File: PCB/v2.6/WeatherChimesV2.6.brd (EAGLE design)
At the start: 102.8 x 78.9 mm, 31 parts, among them U1 MS5803-02BA, X4 BQ24074

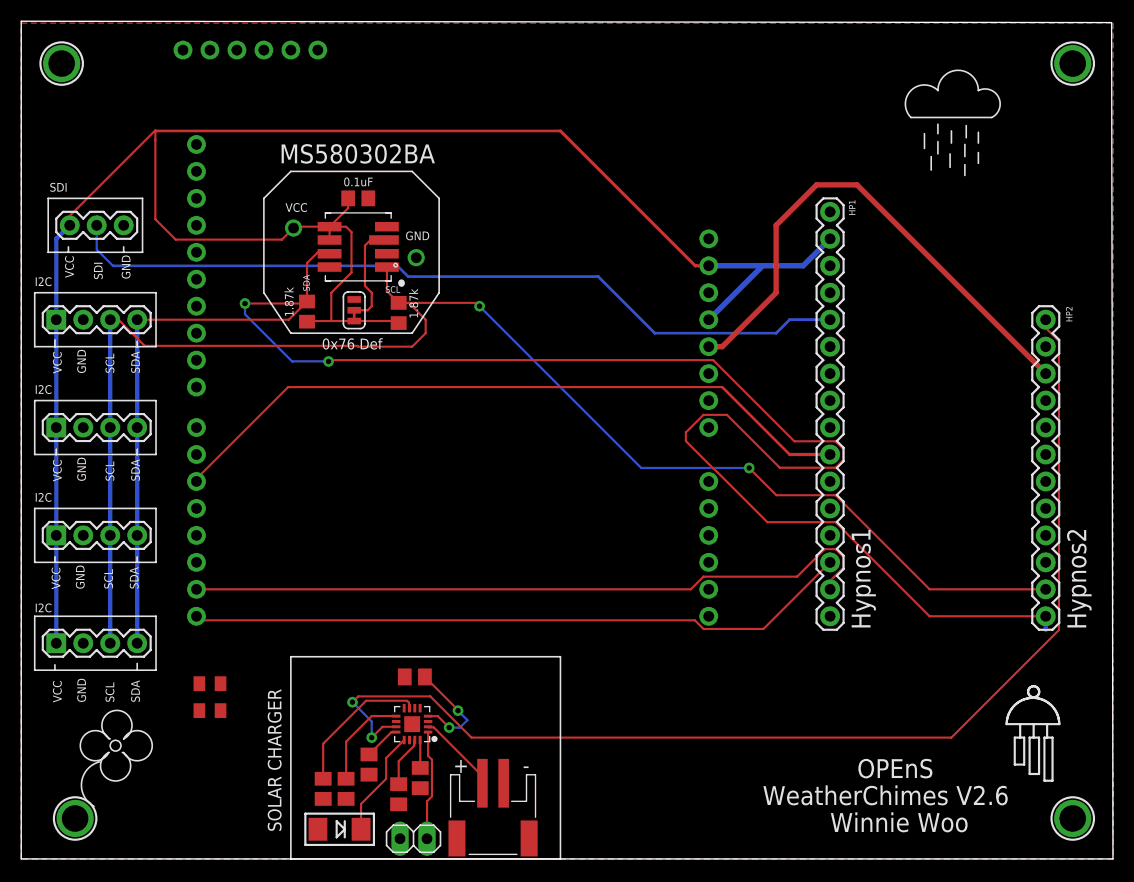
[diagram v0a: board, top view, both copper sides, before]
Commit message: Add files via upload
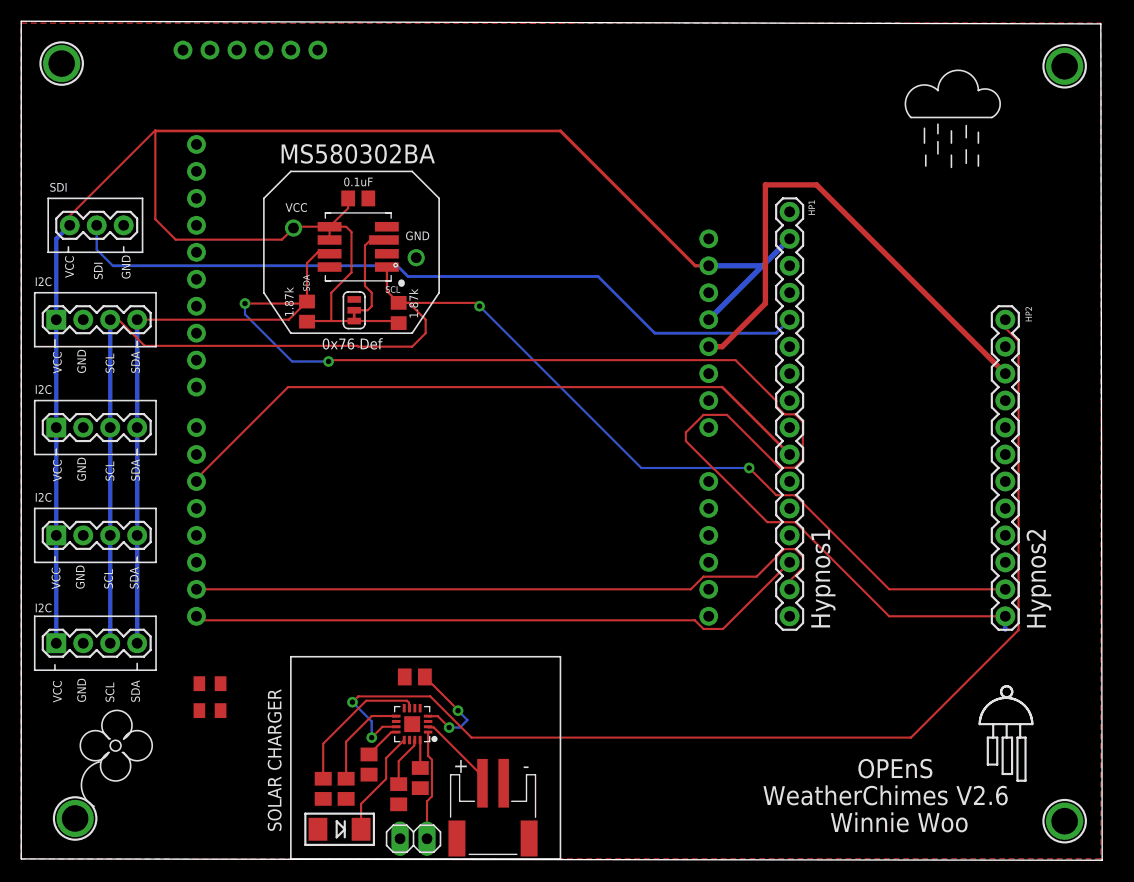
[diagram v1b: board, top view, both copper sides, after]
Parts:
- moved HP1 3.81 mm to (71.1, 62.2)
- moved HP2 3.81 mm to (91.4, 52.1)
- moved U$4 0.80 mm to (97.0, 75.9)
- moved U$5 0.80 mm to (97.0, 4.83)
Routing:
- net SDA: track 183.8 -> 174.1 mm
- net VCC: track 180.2 -> 176.4 mm
- net VBAT: track 109.2 -> 105.4 mm
- net SDI: track 75.9 -> 72.1 mm
- net SCL: track 141.3 -> 137.4 mm
- net RX: track 62.2 -> 58.4 mm
- net 4GONOFF: track 66.2 -> 62.3 mm
- net TX: track 66.4 -> 62.6 mm
- net 5VRAIL: track 49.1 -> 48.2 mm
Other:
- board size 102.8 x 78.9 mm -> 101.8 x 79 mm
